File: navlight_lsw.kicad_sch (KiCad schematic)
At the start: 7 parts, among them U15 TPS26400PWP

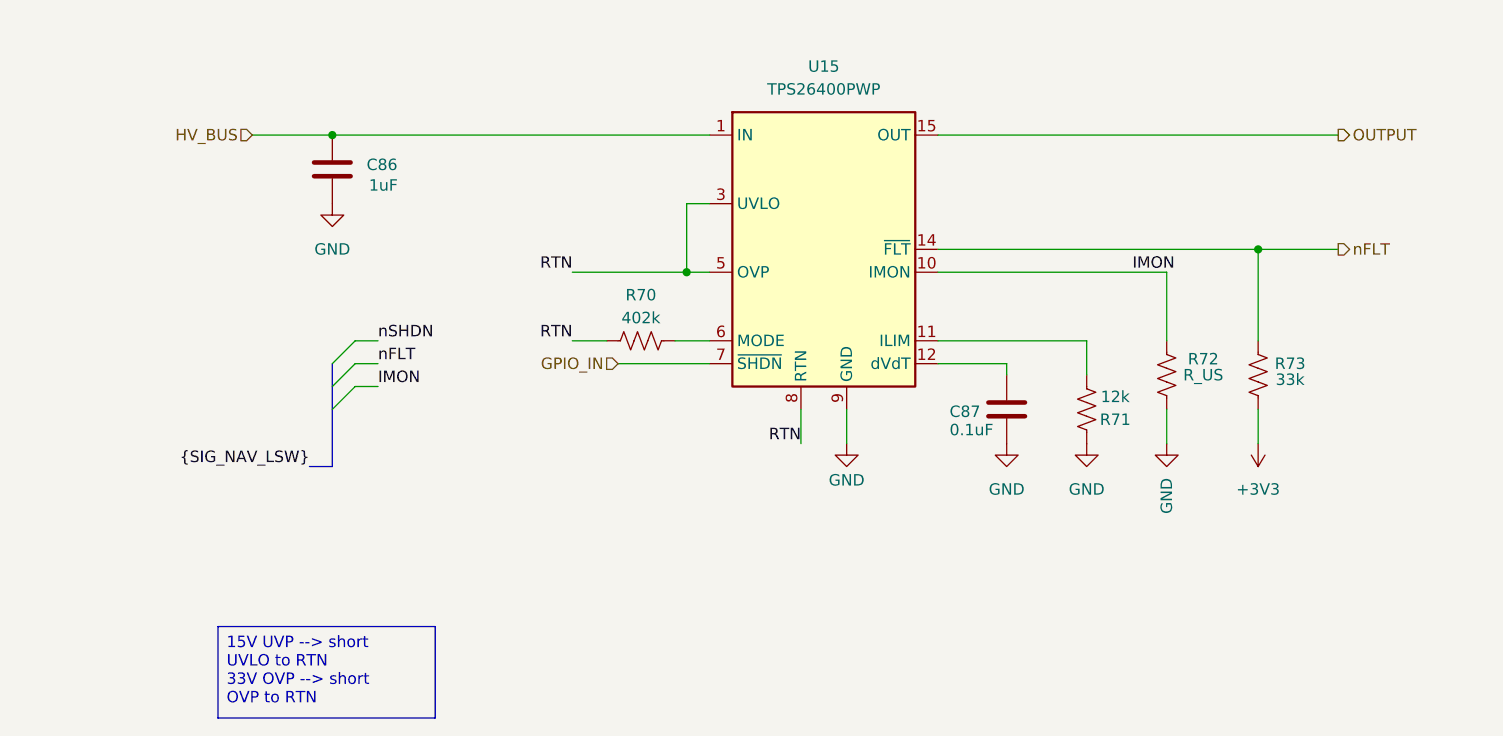
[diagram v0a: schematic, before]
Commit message: Working on it
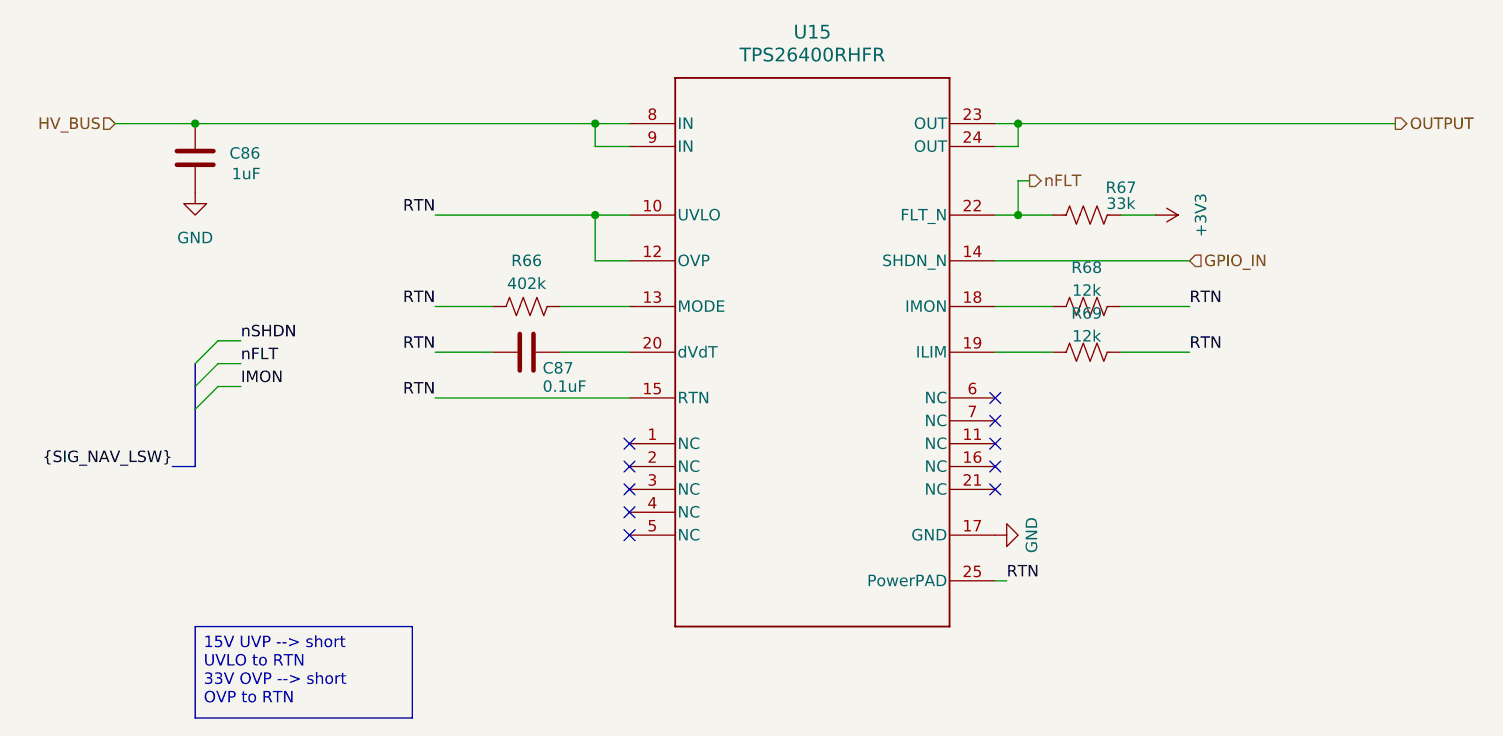
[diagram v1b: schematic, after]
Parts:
- removed R70: 402k, Resistor_SMD:R_0603_1608Metric, symbol Device:R_US
- removed R71: 12k, Resistor_SMD:R_0603_1608Metric, symbol Device:R_US
- removed R72: R_US, Resistor_SMD:R_0603_1608Metric, symbol Device:R_US
- removed R73: 33k, Resistor_SMD:R_0603_1608Metric, symbol Device:R_US
- removed U15: TPS26400PWP, Package_DFN_QFN:VQFN-24-1EP_4x4mm_P0.5mm_EP2.45x2.45mm_ThermalVias, symbol Power_Management:TPS26400PWP
- added R66: 402k, Resistor_SMD:R_0603_1608Metric, symbol Device:R_US
- added R67: 33k, Resistor_SMD:R_0603_1608Metric, symbol Device:R_US
- added R68, R69: 12k, Resistor_SMD:R_0603_1608Metric, symbol Device:R_US
- added U15: TPS26400RHFR, _PowerBoard:RHF0024A-MFG, symbol _TPS26400RHFR:TPS26400RHFR
- C87: Supplier_2 (none) -> JLCPCB; Supplier_2_Price @ QTY (none) -> 1
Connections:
- net +3V3: now also R67.1
- net GND: now also U15.17 (GND); no longer C87.2
- net GPIO_IN: now also U15.14 (SHDN_N)
- net HV_BUS: now also U15.8 (IN), U15.9 (IN)
- net OUTPUT: now also U15.23 (OUT), U15.24 (OUT)
- net RTN: now also C87.1, R66.1, R68.1, R69.1, U15.10 (UVLO), U15.12 (OVP), U15.15 (RTN), U15.25 (PowerPAD)
- net nFLT: now also R67.2, U15.22 (FLT_N)
- new net: R69.2, U15.19 (ILIM)
- new net: R66.2, U15.13 (MODE)
- new net: C87.2, U15.20 (dVdT)
- new net: R68.2, U15.18 (IMON)
- no-connect marks 0 -> 10
